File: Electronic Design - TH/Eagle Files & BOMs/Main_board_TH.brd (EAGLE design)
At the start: 98 x 147 mm, 53 parts, among them M1 ARDUINO-NANO-3.0, Q1 IRF9520, Q2 IRF9520

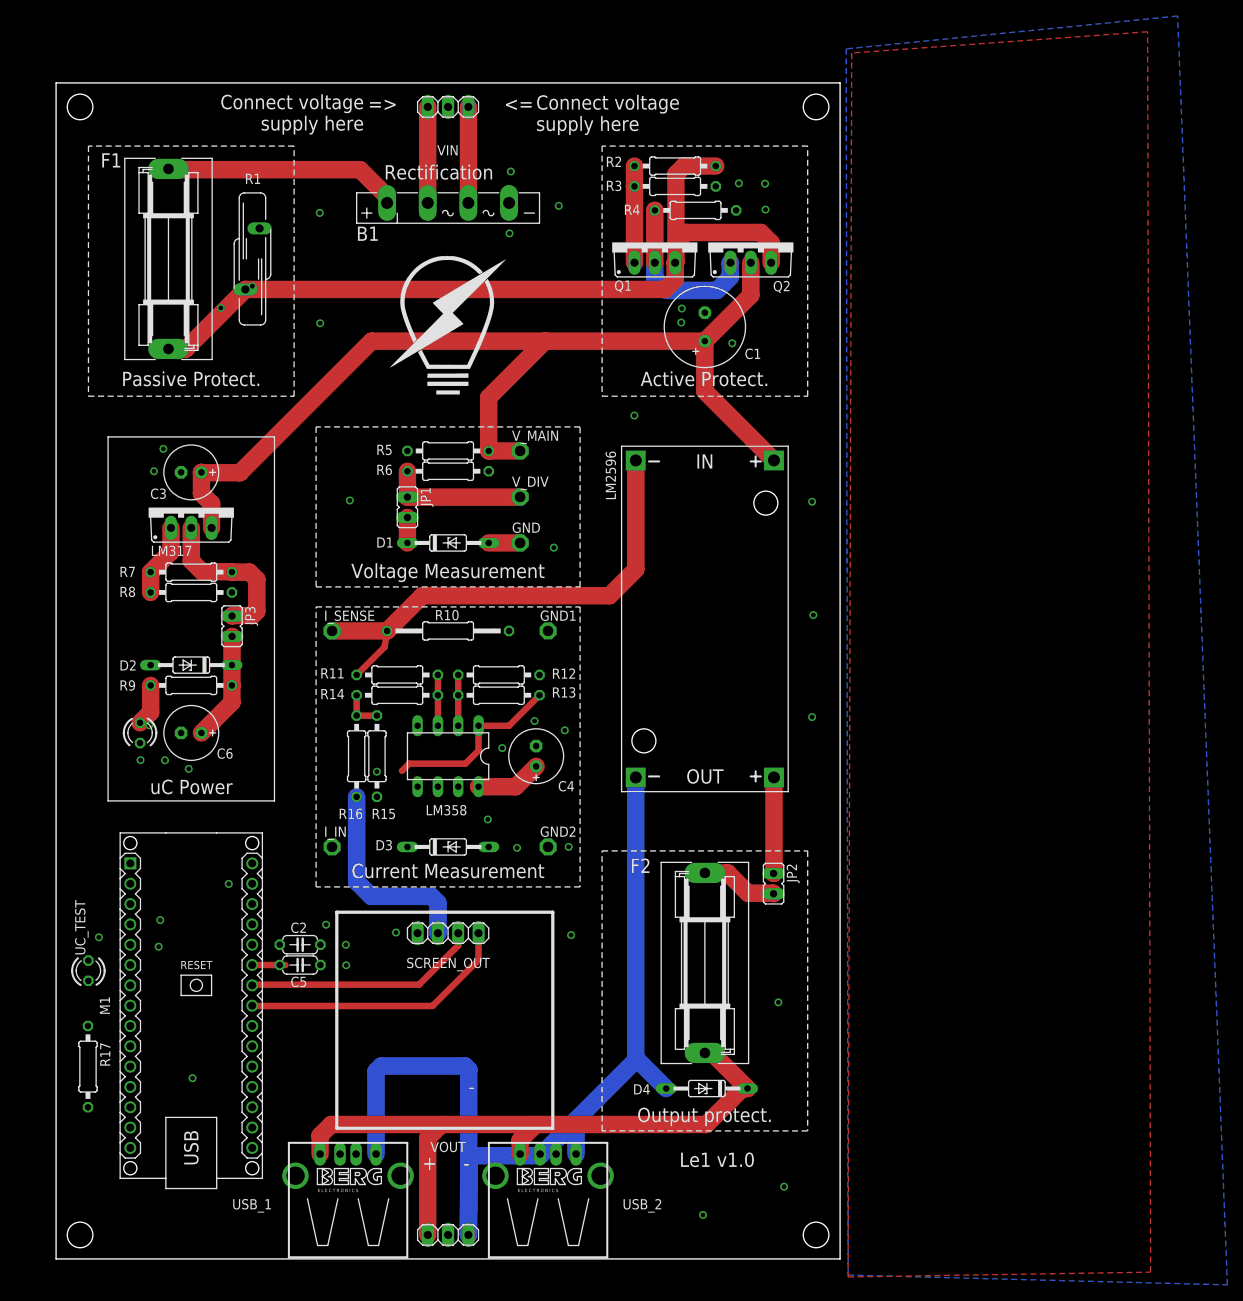
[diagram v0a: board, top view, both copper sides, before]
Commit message: finishing routing
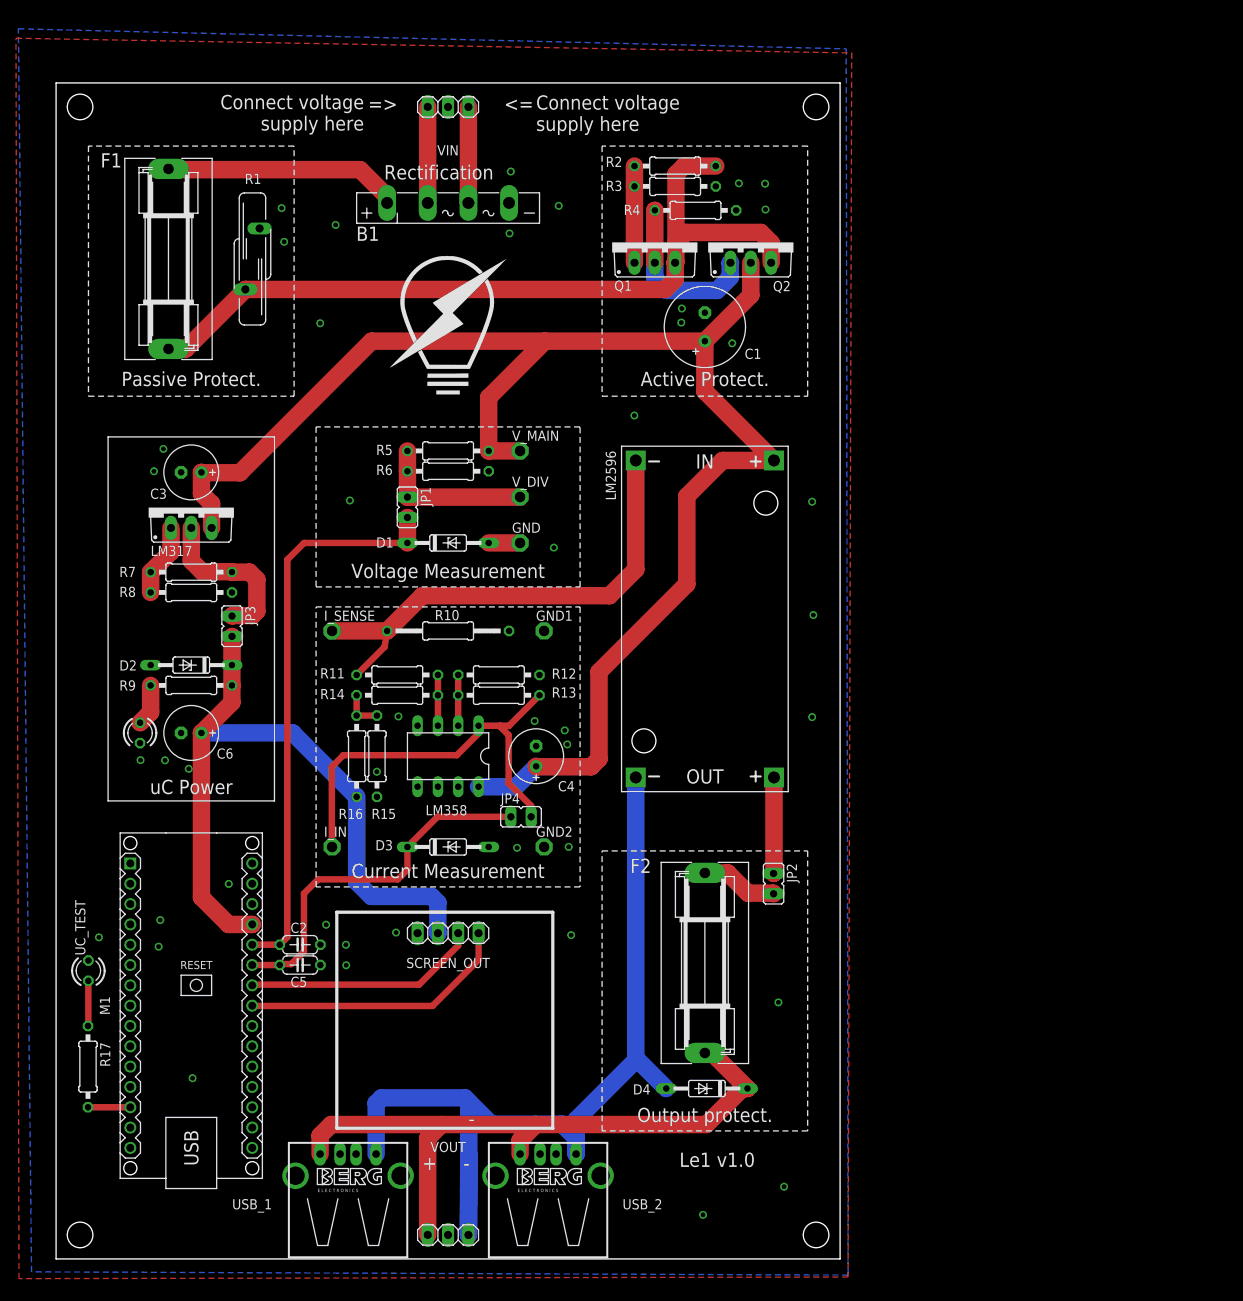
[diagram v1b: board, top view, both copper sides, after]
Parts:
- added JP4: (no value), jumper:JP1
- moved GND1 0.50 mm to (61.0, 78.5)
- moved GND2 0.50 mm to (61.0, 51.5)
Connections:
- removed net GND.1: M1.J1.4
- new net I_IN_PRE: I_IN.TP, JP4.2, LM358.1, R13.1
- net GND: now also M1.J1.4
- net I_IN: now also JP4.1; no longer I_IN.TP, LM358.1, R13.1
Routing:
- net V_IN: track 3.18 -> 71.0 mm
- net VIN_PROTECTED: track 136.7 -> 195.1 mm
- net I_IN_PRE: track 0.00 -> 53.3 mm
- net +5V: track 39.3 -> 90.3 mm
- net I_IN: track 27.1 -> 45.9 mm
- net N$10: track 123.7 -> 117.8 mm
- net N$14: track 0.00 -> 5.66 mm
- net N$13: track 0.00 -> 5.29 mm
- net N$17: track 17.3 -> 19.9 mm
- net GND: vias 45 -> 44
